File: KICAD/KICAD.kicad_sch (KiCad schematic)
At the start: 2327 parts, among them J3 Conn_02x20_Odd_Even, J4 Conn_01x02_Pin, J5 PJ-102A

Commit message: .
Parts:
- removed D2305, D2306, D2307, D2308, D2309, D2310, D2311, D2312, D2313, D2314, D2315, D2316, D2317, D2318, D2319, D2320, D2321, D2322, D2323, D2324, D2325, D2326, D2327, D2328, D2329, D2330, D2331, D2332, D2333, D2334, D2335, D2336, D2337, D2338, D2339, D2340, D2341, D2342, D2343, D2344, D2345, D2346, D2347, D2348, D2349, D2350, D2351, D2352, D2369, D2370, D2371, D2372, D2373, D2374, D2375, D2376, D2377, D2378, D2379, D2380, D2381, D2382, D2383, D2384, D2385, D2386, D2387, D2388, D2389, D2390, D2391, D2392, D2393, D2394, D2395, D2396, D2397, D2398, D2399, D2400, D2401, D2402, D2403, D2404, D2405, D2406, D2407, D2408, D2409, D2410, D2411, D2412, D2413, D2414, D2415, D2416, D2433, D2434, D2435, D2436, D2437, D2438, D2439, D2440, D2441, D2442, D2443, D2444, D2445, D2446, D2447, D2448, D2449, D2450, D2451, D2452, D2453, D2454, D2455, D2456, D2457, D2458, D2459, D2460, D2461, D2462, D2463, D2464, D2465, D2466, D2467, D2468, D2469, D2470, D2471, D2472, D2473, D2474, D2475, D2476, D2477, D2478, D2479, D2480, D2497, D2498, D2499, D2500, D2501, D2502, D2503, D2504, D2505, D2506, D2507, D2508, D2509, D2510, D2511, D2512, D2513, D2514, D2515, D2516, D2517, D2518, D2519, D2520, D2521, D2522, D2523, D2524, D2525, D2526, D2527, D2528, D2529, D2530, D2531, D2532, D2533, D2534, D2535, D2536, D2537, D2538, D2539, D2540, D2541, D2542, D2543, D2544, D2561, D2562, D2563, D2564, D2565, D2566, D2567, D2568, D2569, D2570, D2571, D2572, D2573, D2574, D2575, D2576, D2577, D2578, D2579, D2580, D2581, D2582, D2583, D2584, D2585, D2586, D2587, D2588, D2589, D2590, D2591, D2592, D2593, D2594, D2595, D2596, D2597, D2598, D2599, D2600, D2601, D2602, D2603, D2604, D2605, D2606, D2607, D2608, D2625, D2626, D2627, D2628, D2629, D2630, D2631, D2632, D2633, D2634, D2635, D2636, D2637, D2638, D2639, D2640, D2641, D2642, D2643, D2644, D2645, D2646, D2647, D2648, D2649, D2650, D2651, D2652, D2653, D2654, D2655, D2656, D2657, D2658, D2659, D2660, D2661, D2662, D2663, D2664, D2665, D2666, D2667, D2668, D2669, D2670, D2671, D2672, D2689, D2690, D2691, D2692, D2693, D2694, D2695, D2696, D2697, D2698, D2699, D2700, D2701, D2702, D2703, D2704, D2705, D2706, D2707, D2708, D2709, D2710, D2711, D2712, D2713, D2714, D2715, D2716, D2717, D2718, D2719, D2720, D2721, D2722, D2723, D2724, D2725, D2726, D2727, D2728, D2729, D2730, D2731, D2732, D2733, D2734, D2735, D2736, D2753, D2754, D2755, D2756, D2757, D2758, D2759, D2760, D2761, D2762, D2763, D2764, D2765, D2766, D2767, D2768, D2769, D2770, D2771, D2772, D2773, D2774, D2775, D2776, D2777, D2778, D2779, D2780, D2781, D2782, D2783, D2784, D2785, D2786, D2787, D2788, D2789, D2790, D2791, D2792, D2793, D2794, D2795, D2796, D2797, D2798, D2799, D2800, D2817, D2818, D2819, D2820, D2821, D2822, D2823, D2824, D2825, D2826, D2827, D2828, D2829, D2830, D2831, D2832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: WS2812B, LED_SMD:LED_WS2812B_PLCC4_5.0x5.0mm_P3.2mm, symbol LED:WS2812B
- removed J3: Conn_02x20_Odd_Even, Connector_IDC:IDC-Header_2x20_P2.54mm_Vertical_SMD, symbol Connector_Generic:Conn_02x20_Odd_Even
- added D1009, D1010, D1011, D1012, D1013, D1014, D1015, D1016, D1017, D1018, D1019, D1020, D1021, D1022, D1023, D1024, D1073, D1074, D1075, D1076, D1077, D1078, D1079, D1080, D1081, D1082, D1083, D1084, D1085, D1086, D1087, D1088, D113, D1137, D1138, D1139, D114, D1140, D1141, D1142, D1143, D1144, D1145, D1146, D1147, D1148, D1149, D115, D1150, D1151, D1152, D116, D117, D118, D119, D120, D1201, D1202, D1203, D1204, D1205, D1206, D1207, D1208, D1209, D121, D1210, D1211, D1212, D1213, D1214, D1215, D1216, D122, D123, D124, D125, D126, D1265, D1266, D1267, D1268, D1269, D127, D1270, D1271, D1272, D1273, D1274, D1275, D1276, D1277, D1278, D1279, D128, D1280, D1329, D1330, D1331, D1332, D1333, D1334, D1335, D1336, D1337, D1338, D1339, D1340, D1341, D1342, D1343, D1344, D1393, D1394, D1395, D1396, D1397, D1398, D1399, D1400, D1401, D1402, D1403, D1404, D1405, D1406, D1407, D1408, D1457, D1458, D1459, D1460, D1461, D1462, D1463, D1464, D1465, D1466, D1467, D1468, D1469, D1470, D1471, D1472, D1521, D1522, D1523, D1524, D1525, D1526, D1527, D1528, D1529, D1530, D1531, D1532, D1533, D1534, D1535, D1536, D1585, D1586, D1587, D1588, D1589, D1590, D1591, D1592, D1593, D1594, D1595, D1596, D1597, D1598, D1599, D1600, D1649, D1650, D1651, D1652, D1653, D1654, D1655, D1656, D1657, D1658, D1659, D1660, D1661, D1662, D1663, D1664, D1713, D1714, D1715, D1716, D1717, D1718, D1719, D1720, D1721, D1722, D1723, D1724, D1725, D1726, D1727, D1728, D177, D1777, D1778, D1779, D178, D1780, D1781, D1782, D1783, D1784, D1785, D1786, D1787, D1788, D1789, D179, D1790, D1791, D1792, D180, D181, D182, D183, D184, D1841, D1842, D1843, D1844, D1845, D1846, D1847, D1848, D1849, D185, D1850, D1851, D1852, D1853, D1854, D1855, D1856, D186, D187, D188, D189, D190, D1905, D1906, D1907, D1908, D1909, D191, D1910, D1911, D1912, D1913, D1914, D1915, D1916, D1917, D1918, D1919, D192, D1920, D1969, D1970, D1971, D1972, D1973, D1974, D1975, D1976, D1977, D1978, D1979, D1980, D1981, D1982, D1983, D1984, D2033, D2034, D2035, D2036, D2037, D2038, D2039, D2040, D2041, D2042, D2043, D2044, D2045, D2046, D2047, D2048, D2097, D2098, D2099, D2100, D2101, D2102, D2103, D2104, D2105, D2106, D2107, D2108, D2109, D2110, D2111, D2112, D2161, D2162, D2163, D2164, D2165, D2166, D2167, D2168, D2169, D2170, D2171, D2172, D2173, D2174, D2175, D2176, D2225, D2226, D2227, D2228, D2229, D2230, D2231, D2232, D2233, D2234, D2235, D2236, D2237, D2238, D2239, D2240, D2289, D2290, D2291, D2292, D2293, D2294, D2295, D2296, D2297, D2298, D2299, D2300, D2301, D2302, D2303, D2304, D241, D242, D243, D244, D245, D246, D247, D248, D249, D250, D251, D252, D253, D254, D255, D256, D305, D306, D307, D308, D309, D310, D311, D312, D313, D314, D315, D316, D317, D318, D319, D320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: WS2812B, LED_SMD:LED_WS2812B_PLCC4_5.0x5.0mm_P3.2mm, symbol LED:WS2812B
- added J3: Conn_02x25_Odd_Even, Connector_IDC:IDC-Header_2x25_P2.54mm_Vertical_SMD, symbol Connector_Generic:Conn_02x25_Odd_Even
- C1: footprint Capacitor_SMD:C_0603_1608Metric -> Capacitor_SMD:C_0402_1005Metric
- J5: footprint digikey-footprints:Barrel_Jack_5.5mmODx2.1mmID_PJ-102A -> Connector_BarrelJack:BarrelJack_Wuerth_694102107102_1.0x3.9mm
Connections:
- net BURST_A2 is gone; now on an unnamed net: D9.4 (DIN)
- net BURST_A3 is gone; now on an unnamed net: D17.4 (DIN)
- net BURST_A4 is gone; now on an unnamed net: D25.4 (DIN)
- net BURST_A5 is gone; now on an unnamed net: D33.4 (DIN)
- net BURST_A6 is gone; now on an unnamed net: D41.4 (DIN)
- net BURST_B5 is gone; now on an unnamed net: D545.4 (DIN)
- net BURST_B6 is gone; now on an unnamed net: D553.4 (DIN)
- net BURST_C3 is gone; now on an unnamed net: D1041.4 (DIN)
- net BURST_C4 is gone; now on an unnamed net: D1049.4 (DIN)
- net BURST_D2 is gone; now on an unnamed net: D1545.4 (DIN)
- net BURST_D3 is gone; now on an unnamed net: D1553.4 (DIN)
- net BURST_D4 is gone; now on an unnamed net: D1561.4 (DIN)
- net BURST_D6 is gone; now on an unnamed net: D1577.4 (DIN)
- net BURST_E2 is gone; now on an unnamed net: D2057.4 (DIN)
- net BURST_E4 is gone; now on an unnamed net: D2073.4 (DIN)
- net BURST_E5 is gone; now on an unnamed net: D2081.4 (DIN)
- net BURST_E6 is gone; now on an unnamed net: D2089.4 (DIN)
- net GND: now also D1009.3 (VSS), D1010.3 (VSS), D1011.3 (VSS), D1012.3 (VSS), D1013.3 (VSS), D1014.3 (VSS), D1015.3 (VSS), D1016.3 (VSS), D1017.3 (VSS), D1018.3 (VSS), D1019.3 (VSS), D1020.3 (VSS)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
- net VCC_3: now also D1009.1 (VDD), D1010.1 (VDD), D1011.1 (VDD), D1012.1 (VDD), D1013.1 (VDD), D1014.1 (VDD), D1015.1 (VDD), D1016.1 (VDD), D1017.1 (VDD), D1018.1 (VDD), D1019.1 (VDD), D1020.1 (VDD)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
- net at D1136.2 (DOUT): now also D1137.4 (DIN); no longer D1135.4 (DIN)
- net at D1072.2 (DOUT): now also D1073.4 (DIN); no longer D1136.4 (DIN)
- net at D1897.2 (DOUT): now also D1898.4 (DIN); no longer D1961.4 (DIN)
- net at D1897.4 (DIN): now also D1896.2 (DOUT); no longer D1898.2 (DOUT)
- net at D740.4 (DIN): now also D739.2 (DOUT); no longer D741.2 (DOUT)
- net at D742.2 (DOUT): now also D743.4 (DIN); no longer D741.4 (DIN)
- net at D364.4 (DIN): now also D363.2 (DOUT); no longer D365.2 (DOUT)
- net at D365.4 (DIN): now also D364.2 (DOUT); no longer D366.2 (DOUT)
- net at D1772.4 (DIN): now also D1771.2 (DOUT); no longer D1773.2 (DOUT)
- net at D1773.4 (DIN): now also D1772.2 (DOUT); no longer D1774.2 (DOUT)
- net at D607.2 (DOUT): now also D608.4 (DIN); no longer D606.4 (DIN)
- net at D607.4 (DIN): now also D606.2 (DOUT); no longer D608.2 (DOUT)
- net at D2270.4 (DIN): now also D2269.2 (DOUT); no longer D2271.2 (DOUT)
- net at D2272.2 (DOUT): now also D2273.4 (DIN); no longer D2271.4 (DIN)
- net at D2153.2 (DOUT): now also D2154.4 (DIN); no longer D2217.4 (DIN)
- net at D2153.4 (DIN): now also D2152.2 (DOUT); no longer D2154.2 (DOUT)
- net at D1740.2 (DOUT): now also D1741.4 (DIN); no longer D1739.4 (DIN)
- net at D1740.4 (DIN): now also D1739.2 (DOUT); no longer D1741.2 (DOUT)
- net at D665.4 (DIN): now also D664.2 (DOUT); no longer D601.2 (DOUT)
- net at D601.4 (DIN): now also D600.2 (DOUT); no longer D602.2 (DOUT)
- net at D100.2 (DOUT): now also D101.4 (DIN); no longer D99.4 (DIN)
- net at D101.2 (DOUT): now also D102.4 (DIN); no longer D100.4 (DIN)
- net at D1816.2 (DOUT): now also D1817.4 (DIN); no longer D1880.4 (DIN)
- net at D727.2 (DOUT): now also D728.4 (DIN); no longer D726.4 (DIN)
- net at D727.4 (DIN): now also D726.2 (DOUT); no longer D728.2 (DOUT)
- net at D1863.4 (DIN): now also D1862.2 (DOUT); no longer D1864.2 (DOUT)
- net at D1800.2 (DOUT): now also D1801.4 (DIN); no longer D1864.4 (DIN)
- net at D1874.2 (DOUT): now also D1875.4 (DIN); no longer D1873.4 (DIN)
- net at D1874.4 (DIN): now also D1873.2 (DOUT); no longer D1875.2 (DOUT)
- net at D196.2 (DOUT): now also D197.4 (DIN); no longer D195.4 (DIN)
- net at D197.2 (DOUT): now also D198.4 (DIN); no longer D196.4 (DIN)
- net at D2022.4 (DIN): now also D2021.2 (DOUT); no longer D2023.2 (DOUT)
- net at D2023.4 (DIN): now also D2022.2 (DOUT); no longer D2024.2 (DOUT)
- net at D617.4 (DIN): now also D616.2 (DOUT); no longer D618.2 (DOUT)
- net at D619.2 (DOUT): now also D620.4 (DIN); no longer D618.4 (DIN)
- net at D609.2 (DOUT): now also D610.4 (DIN); no longer D673.4 (DIN)
- net at D981.4 (DIN): now also D980.2 (DOUT); no longer D982.2 (DOUT)
- net at D982.4 (DIN): now also D981.2 (DOUT); no longer D983.2 (DOUT)
- net at D593.2 (DOUT): now also D594.4 (DIN); no longer D657.4 (DIN)
- net at D593.4 (DIN): now also D592.2 (DOUT); no longer D594.2 (DOUT)
- net at D905.4 (DIN): now also D904.2 (DOUT); no longer D841.2 (DOUT)
- net at D841.4 (DIN): now also D840.2 (DOUT); no longer D842.2 (DOUT)
- net at D1863.2 (DOUT): now also D1864.4 (DIN); no longer D1862.4 (DIN)
- net at D1387.2 (DOUT): now also D1388.4 (DIN); no longer D1386.4 (DIN)
- net at D1387.4 (DIN): now also D1386.2 (DOUT); no longer D1388.2 (DOUT)
- net at D230.2 (DOUT): now also D231.4 (DIN); no longer D229.4 (DIN)
- net at D231.2 (DOUT): now also D232.4 (DIN); no longer D230.4 (DIN)
- net at D860.4 (DIN): now also D859.2 (DOUT); no longer D861.2 (DOUT)
- net at D862.2 (DOUT): now also D863.4 (DIN); no longer D861.4 (DIN)
- net BURST_A1 renamed BURST_1
- net BURST_B3 renamed BURST_12
- net BURST_C5 renamed BURST_23
- net BURST_D1 renamed BURST_33
- net BURST_E3 renamed BURST_44
- new net: D1915.2 (DOUT), D1916.4 (DIN)
- new net: D1914.2 (DOUT), D1915.4 (DIN)
- new net: D441.2 (DOUT), D442.4 (DIN)
- new net: D440.2 (DOUT), D441.4 (DIN)
- new net: D1528.2 (DOUT), D1529.4 (DIN)
- new net: D1527.2 (DOUT), D1528.4 (DIN)
- new net: D435.2 (DOUT), D436.4 (DIN)
- new net: D434.2 (DOUT), D435.4 (DIN)
- new net: D694.2 (DOUT), D695.4 (DIN)
- new net: D693.2 (DOUT), D694.4 (DIN)
- new net: D2175.2 (DOUT), D2176.4 (DIN)
- new net: D2174.2 (DOUT), D2175.4 (DIN)
- new net: D628.2 (DOUT), D629.4 (DIN)
- new net: D627.2 (DOUT), D628.4 (DIN)
- new net: D1784.2 (DOUT), D1785.4 (DIN)
- new net: D1783.2 (DOUT), D1784.4 (DIN)
- new net: D2173.2 (DOUT), D2174.4 (DIN)
- new net: D2172.2 (DOUT), D2173.4 (DIN)
- new net: D1335.2 (DOUT), D1336.4 (DIN)
- new net: D1334.2 (DOUT), D1335.4 (DIN)
- new net: D509.2 (DOUT), D510.4 (DIN)
- new net: D508.2 (DOUT), D509.4 (DIN)
- new net: D433.2 (DOUT), D434.4 (DIN)
- new net: D49.2 (DOUT), D50.4 (DIN)
- new net: D1336.2 (DOUT), D1337.4 (DIN)
- new net: D1274.2 (DOUT), D1275.4 (DIN)
- new net: D1273.2 (DOUT), D1274.4 (DIN)
- new net: D1592.2 (DOUT), D1593.4 (DIN)
- new net: D1591.2 (DOUT), D1592.4 (DIN)
- new net: D1661.2 (DOUT), D1662.4 (DIN)
- new net: D1660.2 (DOUT), D1661.4 (DIN)
- new net: D1077.2 (DOUT), D1078.4 (DIN)
- new net: D1076.2 (DOUT), D1077.4 (DIN)
- new net: D753.2 (DOUT), D754.4 (DIN)
- new net: D59.2 (DOUT), D60.4 (DIN)
- new net: D58.2 (DOUT), D59.4 (DIN)
- new net: D370.2 (DOUT), D371.4 (DIN)
- new net: D369.2 (DOUT), D370.4 (DIN)
- new net: D1460.2 (DOUT), D1461.4 (DIN)
- new net: D1459.2 (DOUT), D1460.4 (DIN)
- new net: D1981.2 (DOUT), D1982.4 (DIN)
- new net: D1980.2 (DOUT), D1981.4 (DIN)
- new net: D767.2 (DOUT), D768.4 (DIN)
- new net: D766.2 (DOUT), D767.4 (DIN)
- new net: D1269.2 (DOUT), D1270.4 (DIN)
- new net: D1268.2 (DOUT), D1269.4 (DIN)
- new net: D1143.2 (DOUT), D1144.4 (DIN)
- new net: D1142.2 (DOUT), D1143.4 (DIN)
- new net: D1917.2 (DOUT), D1918.4 (DIN)
- new net: D1916.2 (DOUT), D1917.4 (DIN)
- new net: D639.2 (DOUT), D640.4 (DIN)
- new net: D638.2 (DOUT), D639.4 (DIN)
- new net: D1075.2 (DOUT), D1076.4 (DIN)
- new net: D1074.2 (DOUT), D1075.4 (DIN)
- new net: D1588.2 (DOUT), D1589.4 (DIN)
- new net: D1587.2 (DOUT), D1588.4 (DIN)
- new net: D1910.2 (DOUT), D1911.4 (DIN)
- new net: D1909.2 (DOUT), D1910.4 (DIN)
- new net: D1974.2 (DOUT), D1975.4 (DIN)
- new net: D1973.2 (DOUT), D1974.4 (DIN)
- new net: D894.2 (DOUT), D895.4 (DIN)
- new net: D893.2 (DOUT), D894.4 (DIN)
- new net: D1790.2 (DOUT), D1791.4 (DIN)
- new net: D1789.2 (DOUT), D1790.4 (DIN)
- new net: D182.2 (DOUT), D183.4 (DIN)
- new net: D181.2 (DOUT), D182.4 (DIN)
- new net: D1979.2 (DOUT), D1980.4 (DIN)
- new net: D1725.2 (DOUT), D1726.4 (DIN)
- new net: D1724.2 (DOUT), D1725.4 (DIN)
- new net: D2034.2 (DOUT), D2035.4 (DIN)
- new net: D2033.2 (DOUT), D2034.4 (DIN)
- new net: D1139.2 (DOUT), D1140.4 (DIN)
- new net: D1138.2 (DOUT), D1139.4 (DIN)
- new net: D114.2 (DOUT), D115.4 (DIN)
- new net: D113.2 (DOUT), D114.4 (DIN)
- new net: D1785.2 (DOUT), D1786.4 (DIN)
- new net: D500.2 (DOUT), D501.4 (DIN)
- new net: D499.2 (DOUT), D500.4 (DIN)
- new net: D1141.2 (DOUT), D1142.4 (DIN)
- new net: D1140.2 (DOUT), D1141.4 (DIN)
- new net: D507.2 (DOUT), D508.4 (DIN)
- new net: D568.2 (DOUT), D569.4 (DIN)
- new net: D567.2 (DOUT), D568.4 (DIN)
- new net: D881.2 (DOUT), D882.4 (DIN)
- new net: D1202.2 (DOUT), D1203.4 (DIN)
- new net: D1201.2 (DOUT), D1202.4 (DIN)
- new net: D1913.2 (DOUT), D1914.4 (DIN)
- new net: D1912.2 (DOUT), D1913.4 (DIN)
- new net: D820.2 (DOUT), D821.4 (DIN)
- new net: D819.2 (DOUT), D820.4 (DIN)
- new net: D1919.2 (DOUT), D1920.4 (DIN)
- new net: D2292.2 (DOUT), D2293.4 (DIN)
- new net: D2291.2 (DOUT), D2292.4 (DIN)
- new net: D1082.2 (DOUT), D1083.4 (DIN)
- new net: D1081.2 (DOUT), D1082.4 (DIN)
- new net: D243.2 (DOUT), D244.4 (DIN)
- new net: D242.2 (DOUT), D243.4 (DIN)
- new net: D1791.2 (DOUT), D1792.4 (DIN)
- new net: D689.2 (DOUT), D690.4 (DIN)
- new net: D2161.2 (DOUT), D2162.4 (DIN)
- new net: D1599.2 (DOUT), D1600.4 (DIN)
- new net: D1598.2 (DOUT), D1599.4 (DIN)
- new net: D1978.2 (DOUT), D1979.4 (DIN)
- new net: D1977.2 (DOUT), D1978.4 (DIN)
- new net: D1367.2 (DOUT), D1368.4 (DIN)
- new net: D762.2 (DOUT), D763.4 (DIN)
- new net: D761.2 (DOUT), D762.4 (DIN)
- new net: D2231.2 (DOUT), D2232.4 (DIN)
- new net: D2230.2 (DOUT), D2231.4 (DIN)
- new net: D1457.2 (DOUT), D1458.4 (DIN)
- new net: D1456.2 (DOUT), D1457.4 (DIN)
- new net: D1659.2 (DOUT), D1660.4 (DIN)
- new net: D1401.2 (DOUT), D1402.4 (DIN)
- new net: D1400.2 (DOUT), D1401.4 (DIN)
- new net: D888.2 (DOUT), D889.4 (DIN)
- new net: D887.2 (DOUT), D888.4 (DIN)
- new net: D191.2 (DOUT), D192.4 (DIN)
- new net: D190.2 (DOUT), D191.4 (DIN)
- new net: D1972.2 (DOUT), D1973.4 (DIN)
- new net: D631.2 (DOUT), D632.4 (DIN)
- new net: D630.2 (DOUT), D631.4 (DIN)
- new net: D1151.2 (DOUT), D1152.4 (DIN)
- new net: D1150.2 (DOUT), D1151.4 (DIN)
- new net: D1652.2 (DOUT), D1653.4 (DIN)
- new net: D1651.2 (DOUT), D1652.4 (DIN)
- new net: D377.2 (DOUT), D378.4 (DIN)
- new net: D376.2 (DOUT), D377.4 (DIN)
- new net: D1727.2 (DOUT), D1728.4 (DIN)
- new net: D1726.2 (DOUT), D1727.4 (DIN)
- new net: D700.2 (DOUT), D701.4 (DIN)
- new net: D699.2 (DOUT), D700.4 (DIN)
- new net: D51.2 (DOUT), D52.4 (DIN)
- new net: D50.2 (DOUT), D51.4 (DIN)
- new net: D255.2 (DOUT), D256.4 (DIN)
- new net: D254.2 (DOUT), D255.4 (DIN)
- new net: D572.2 (DOUT), D573.4 (DIN)
- new net: D571.2 (DOUT), D572.4 (DIN)
- new net: D2301.2 (DOUT), D2302.4 (DIN)
- new net: D2300.2 (DOUT), D2301.4 (DIN)
- new net: D245.2 (DOUT), D246.4 (DIN)
- new net: D244.2 (DOUT), D245.4 (DIN)
- new net: D1276.2 (DOUT), D1277.4 (DIN)
- new net: D1275.2 (DOUT), D1276.4 (DIN)
- new net: D252.2 (DOUT), D253.4 (DIN)
- new net: D251.2 (DOUT), D252.4 (DIN)
- new net: D946.2 (DOUT), D947.4 (DIN)
- new net: D945.2 (DOUT), D946.4 (DIN)
- new net: D2038.2 (DOUT), D2039.4 (DIN)
- new net: D2037.2 (DOUT), D2038.4 (DIN)
- new net: D1396.2 (DOUT), D1397.4 (DIN)
- new net: D1395.2 (DOUT), D1396.4 (DIN)
- new net: D1969.2 (DOUT), D1970.4 (DIN)
- new net: D317.2 (DOUT), D318.4 (DIN)
- new net: D316.2 (DOUT), D317.4 (DIN)
- new net: D1085.2 (DOUT), D1086.4 (DIN)
- new net: D1084.2 (DOUT), D1085.4 (DIN)
- new net: D1786.2 (DOUT), D1787.4 (DIN)
- new net: D1533.2 (DOUT), D1534.4 (DIN)
- new net: D1532.2 (DOUT), D1533.4 (DIN)
- new net: D1653.2 (DOUT), D1654.4 (DIN)
- new net: D574.2 (DOUT), D575.4 (DIN)
- new net: D573.2 (DOUT), D574.4 (DIN)
- new net: D702.2 (DOUT), D703.4 (DIN)
- new net: D701.2 (DOUT), D702.4 (DIN)
- new net: D320.2 (DOUT), D321.4 (DIN)
- new net: D319.2 (DOUT), D320.4 (DIN)
- new net: D1018.2 (DOUT), D1019.4 (DIN)
- new net: D1017.2 (DOUT), D1018.4 (DIN)
- new net: D1777.2 (DOUT), D1778.4 (DIN)
- new net: D634.2 (DOUT), D635.4 (DIN)
- new net: D633.2 (DOUT), D634.4 (DIN)
- new net: D379.2 (DOUT), D380.4 (DIN)
- new net: D378.2 (DOUT), D379.4 (DIN)
- new net: D188.2 (DOUT), D189.4 (DIN)
- new net: D187.2 (DOUT), D188.4 (DIN)
- new net: D1011.2 (DOUT), D1012.4 (DIN)
- new net: D1010.2 (DOUT), D1011.4 (DIN)
- new net: D502.2 (DOUT), D503.4 (DIN)
- new net: D501.2 (DOUT), D502.4 (DIN)
- new net: D2035.2 (DOUT), D2036.4 (DIN)
- new net: D1535.2 (DOUT), D1536.4 (DIN)
- new net: D1083.2 (DOUT), D1084.4 (DIN)
- new net: D1713.2 (DOUT), D1714.4 (DIN)
- new net: D1023.2 (DOUT), D1024.4 (DIN)
- new net: D1022.2 (DOUT), D1023.4 (DIN)
- new net: D2110.2 (DOUT), D2111.4 (DIN)
- new net: D2109.2 (DOUT), D2110.4 (DIN)
- new net: D1656.2 (DOUT), D1657.4 (DIN)
- new net: D1655.2 (DOUT), D1656.4 (DIN)
- new net: D1342.2 (DOUT), D1343.4 (DIN)
- new net: D1341.2 (DOUT), D1342.4 (DIN)
- new net: D765.2 (DOUT), D766.4 (DIN)
- new net: D764.2 (DOUT), D765.4 (DIN)
- new net: D823.2 (DOUT), D824.4 (DIN)
- new net: D822.2 (DOUT), D823.4 (DIN)
- new net: D1137.2 (DOUT), D1138.4 (DIN)
- new net: D1271.2 (DOUT), D1272.4 (DIN)
- new net: D1270.2 (DOUT), D1271.4 (DIN)
- new net: D307.2 (DOUT), D308.4 (DIN)
- new net: D306.2 (DOUT), D307.4 (DIN)
- new net: D444.2 (DOUT), D445.4 (DIN)
- new net: D443.2 (DOUT), D444.4 (DIN)
- new net: D2162.2 (DOUT), D2163.4 (DIN)
- new net: D1593.2 (DOUT), D1594.4 (DIN)
- new net: D116.2 (DOUT), D117.4 (DIN)
- new net: D115.2 (DOUT), D116.4 (DIN)
- new net: D697.2 (DOUT), D698.4 (DIN)
- new net: D696.2 (DOUT), D697.4 (DIN)
- new net: D57.2 (DOUT), D58.4 (DIN)
- new net: D54.2 (DOUT), D55.4 (DIN)
- new net: D53.2 (DOUT), D54.4 (DIN)
- new net: D1970.2 (DOUT), D1971.4 (DIN)
- new net: D691.2 (DOUT), D692.4 (DIN)
- new net: D690.2 (DOUT), D691.4 (DIN)
- new net: D896.2 (DOUT), D897.4 (DIN)
- new net: D740.2 (DOUT), D741.4 (DIN)
- new net: D1754.2 (DOUT), D1755.4 (DIN)
- new net: D1975.2 (DOUT), D1976.4 (DIN)
- new net: D1339.2 (DOUT), D1340.4 (DIN)
- new net: D1338.2 (DOUT), D1339.4 (DIN)
- new net: D886.2 (DOUT), D887.4 (DIN)
- new net: D885.2 (DOUT), D886.4 (DIN)
- new net: D2108.2 (DOUT), D2109.4 (DIN)
- new net: D2107.2 (DOUT), D2108.4 (DIN)
- new net: D884.2 (DOUT), D885.4 (DIN)
- new net: D2232.2 (DOUT), D2233.4 (DIN)
- new net: D2036.2 (DOUT), D2037.4 (DIN)
- new net: D2236.2 (DOUT), D2237.4 (DIN)
- new net: D2235.2 (DOUT), D2236.4 (DIN)
- new net: D1021.2 (DOUT), D1022.4 (DIN)
- new net: D1842.2 (DOUT), D1843.4 (DIN)
- new net: D1841.2 (DOUT), D1842.4 (DIN)
- new net: D1715.2 (DOUT), D1716.4 (DIN)
- new net: D1714.2 (DOUT), D1715.4 (DIN)
- new net: D1983.2 (DOUT), D1984.4 (DIN)
- new net: D1982.2 (DOUT), D1983.4 (DIN)
- new net: D1337.2 (DOUT), D1338.4 (DIN)
- new net: D569.2 (DOUT), D570.4 (DIN)
- new net: D383.2 (DOUT), D384.4 (DIN)
- new net: D703.2 (DOUT), D704.4 (DIN)
- new net: D1272.2 (DOUT), D1273.4 (DIN)
- new net: D1206.2 (DOUT), D1207.4 (DIN)
- new net: D1205.2 (DOUT), D1206.4 (DIN)
- new net: D52.2 (DOUT), D53.4 (DIN)
- new net: D250.2 (DOUT), D251.4 (DIN)
- new net: D1215.2 (DOUT), D1216.4 (DIN)
- new net: D1214.2 (DOUT), D1215.4 (DIN)
- new net: D511.2 (DOUT), D512.4 (DIN)
- new net: D510.2 (DOUT), D511.4 (DIN)
- new net: D2303.2 (DOUT), D2304.4 (DIN)
- new net: D2302.2 (DOUT), D2303.4 (DIN)
- new net: D305.2 (DOUT), D306.4 (DIN)
- new net: D1531.2 (DOUT), D1532.4 (DIN)
- new net: D1530.2 (DOUT), D1531.4 (DIN)
- new net: D695.2 (DOUT), D696.4 (DIN)
- new net: D1534.2 (DOUT), D1535.4 (DIN)
- new net: D118.2 (DOUT), D119.4 (DIN)
- new net: D117.2 (DOUT), D118.4 (DIN)
- new net: D372.2 (DOUT), D373.4 (DIN)
- new net: D371.2 (DOUT), D372.4 (DIN)
- new net: D1905.2 (DOUT), D1906.4 (DIN)
- new net: D436.2 (DOUT), D437.4 (DIN)
- new net: D1851.2 (DOUT), D1852.4 (DIN)
- new net: D1850.2 (DOUT), D1851.4 (DIN)
- new net: D1403.2 (DOUT), D1404.4 (DIN)
- new net: D1402.2 (DOUT), D1403.4 (DIN)
- new net: D1458.2 (DOUT), D1459.4 (DIN)
- new net: D829.2 (DOUT), D830.4 (DIN)
- new net: D828.2 (DOUT), D829.4 (DIN)
- new net: D1852.2 (DOUT), D1853.4 (DIN)
- new net: D1918.2 (DOUT), D1919.4 (DIN)
- new net: D1986.2 (DOUT), D1987.4 (DIN)
- new net: D763.2 (DOUT), D764.4 (DIN)
- new net: D1657.2 (DOUT), D1658.4 (DIN)
- new net: D1404.2 (DOUT), D1405.4 (DIN)
- new net: D189.2 (DOUT), D190.4 (DIN)
- new net: D382.2 (DOUT), D383.4 (DIN)
- new net: D381.2 (DOUT), D382.4 (DIN)
- new net: D1516.2 (DOUT), D1517.4 (DIN)
- new net: D2105.2 (DOUT), D2106.4 (DIN)
- new net: D2104.2 (DOUT), D2105.4 (DIN)
- new net: D122.2 (DOUT), D123.4 (DIN)
- new net: D121.2 (DOUT), D122.4 (DIN)
- new net: D1662.2 (DOUT), D1663.4 (DIN)
- new net: D1333.2 (DOUT), D1334.4 (DIN)
- new net: D1332.2 (DOUT), D1333.4 (DIN)
- new net: D564.2 (DOUT), D565.4 (DIN)
- new net: D563.2 (DOUT), D564.4 (DIN)
- new net: D180.2 (DOUT), D181.4 (DIN)
- new net: D2295.2 (DOUT), D2296.4 (DIN)
- new net: D2294.2 (DOUT), D2295.4 (DIN)
- new net: D2169.2 (DOUT), D2170.4 (DIN)
- new net: D2168.2 (DOUT), D2169.4 (DIN)
- new net: D2133.2 (DOUT), D2134.4 (DIN)
- new net: D959.2 (DOUT), D960.4 (DIN)
- new net: D958.2 (DOUT), D959.4 (DIN)
- new net: D2045.2 (DOUT), D2046.4 (DIN)
- new net: D2044.2 (DOUT), D2045.4 (DIN)
- new net: D315.2 (DOUT), D316.4 (DIN)
- new net: D314.2 (DOUT), D315.4 (DIN)
- new net: D1279.2 (DOUT), D1280.4 (DIN)
- new net: D1278.2 (DOUT), D1279.4 (DIN)
- new net: D1212.2 (DOUT), D1213.4 (DIN)
- new net: D1211.2 (DOUT), D1212.4 (DIN)
- new net: D1080.2 (DOUT), D1081.4 (DIN)
- new net: D635.2 (DOUT), D636.4 (DIN)
- new net: D751.2 (DOUT), D752.4 (DIN)
- new net: D1213.2 (DOUT), D1214.4 (DIN)
- new net: D445.2 (DOUT), D446.4 (DIN)
- new net: D566.2 (DOUT), D567.4 (DIN)
- new net: D505.2 (DOUT), D506.4 (DIN)
- new net: D504.2 (DOUT), D505.4 (DIN)
- new net: D1506.2 (DOUT), D1507.4 (DIN)
- new net: D1020.2 (DOUT), D1021.4 (DIN)
- new net: D1529.2 (DOUT), D1530.4 (DIN)
- new net: D253.2 (DOUT), D254.4 (DIN)
- new net: D1340.2 (DOUT), D1341.4 (DIN)
- new net: D491.2 (DOUT), D492.4 (DIN)
- new net: D490.2 (DOUT), D491.4 (DIN)
- new net: D1782.2 (DOUT), D1783.4 (DIN)
- new net: D1781.2 (DOUT), D1782.4 (DIN)
- new net: D2234.2 (DOUT), D2235.4 (DIN)
- new net: D2233.2 (DOUT), D2234.4 (DIN)
- new net: D1911.2 (DOUT), D1912.4 (DIN)
- new net: D892.2 (DOUT), D893.4 (DIN)
- new net: D1779.2 (DOUT), D1780.4 (DIN)
- new net: D1778.2 (DOUT), D1779.4 (DIN)
- new net: D2163.2 (DOUT), D2164.4 (DIN)
- new net: D1086.2 (DOUT), D1087.4 (DIN)
- new net: D120.2 (DOUT), D121.4 (DIN)
- new net: D119.2 (DOUT), D120.4 (DIN)
- new net: D994.2 (DOUT), D995.4 (DIN)
- new net: D484.2 (DOUT), D485.4 (DIN)
- new net: D1407.2 (DOUT), D1408.4 (DIN)
- new net: D1406.2 (DOUT), D1407.4 (DIN)
- new net: D2246.2 (DOUT), D2247.4 (DIN)
- new net: D1526.2 (DOUT), D1527.4 (DIN)
- new net: D951.2 (DOUT), D952.4 (DIN)
- new net: D950.2 (DOUT), D951.4 (DIN)
- new net: D61.2 (DOUT), D62.4 (DIN)
- new net: D60.2 (DOUT), D61.4 (DIN)
- new net: D2039.2 (DOUT), D2040.4 (DIN)
- new net: D483.2 (DOUT), D484.4 (DIN)
- new net: D2247.2 (DOUT), D2248.4 (DIN)
- new net: D309.2 (DOUT), D310.4 (DIN)
- new net: D308.2 (DOUT), D309.4 (DIN)
- new net: D876.2 (DOUT), D877.4 (DIN)
- new net: D891.2 (DOUT), D892.4 (DIN)
- new net: D890.2 (DOUT), D891.4 (DIN)
- new net: D1399.2 (DOUT), D1400.4 (DIN)
- new net: D560.2 (DOUT), D561.4 (DIN)
- new net: D152.2 (DOUT), D153.4 (DIN)
- new net: D889.2 (DOUT), D890.4 (DIN)
- new net: D2149.2 (DOUT), D2150.4 (DIN)
- new net: D2226.2 (DOUT), D2227.4 (DIN)
- new net: D2225.2 (DOUT), D2226.4 (DIN)
- new net: D875.2 (DOUT), D876.4 (DIN)
- new net: D2293.2 (DOUT), D2294.4 (DIN)
- new net: D1525.2 (DOUT), D1526.4 (DIN)
- new net: D1524.2 (DOUT), D1525.4 (DIN)
- new net: D1471.2 (DOUT), D1472.4 (DIN)
- new net: D1470.2 (DOUT), D1471.4 (DIN)
- new net: D1898.2 (DOUT), D1899.4 (DIN)
- new net: D56.2 (DOUT), D57.4 (DIN)
- new net: D55.2 (DOUT), D56.4 (DIN)
- new net: D1637.2 (DOUT), D1638.4 (DIN)
- new net: D1370.2 (DOUT), D1371.4 (DIN)
- new net: D620.2 (DOUT), D621.4 (DIN)
- new net: D1788.2 (DOUT), D1789.4 (DIN)
- new net: D1787.2 (DOUT), D1788.4 (DIN)
- new net: D503.2 (DOUT), D504.4 (DIN)
- new net: D1227.2 (DOUT), D1228.4 (DIN)
- new net: D2043.2 (DOUT), D2044.4 (DIN)
- new net: D2042.2 (DOUT), D2043.4 (DIN)
- new net: D947.2 (DOUT), D948.4 (DIN)
- new net: D1087.2 (DOUT), D1088.4 (DIN)
- new net: D882.2 (DOUT), D883.4 (DIN)
- new net: D1720.2 (DOUT), D1721.4 (DIN)
- new net: D1719.2 (DOUT), D1720.4 (DIN)
- new net: D239.2 (DOUT), D240.4 (DIN)
- new net: D437.2 (DOUT), D438.4 (DIN)
- new net: D2099.2 (DOUT), D2100.4 (DIN)
- new net: D2098.2 (DOUT), D2099.4 (DIN)
- new net: D1595.2 (DOUT), D1596.4 (DIN)
- new net: D1594.2 (DOUT), D1595.4 (DIN)
- new net: D953.2 (DOUT), D954.4 (DIN)
- new net: D952.2 (DOUT), D953.4 (DIN)
- new net: D179.2 (DOUT), D180.4 (DIN)
- new net: D178.2 (DOUT), D179.4 (DIN)
- new net: D821.2 (DOUT), D822.4 (DIN)
- new net: D1971.2 (DOUT), D1972.4 (DIN)
- new net: D83.2 (DOUT), D84.4 (DIN)
- new net: D2238.2 (DOUT), D2239.4 (DIN)
- new net: D2237.2 (DOUT), D2238.4 (DIN)
- new net: D2103.2 (DOUT), D2104.4 (DIN)
- new net: D2102.2 (DOUT), D2103.4 (DIN)
- new net: D79.2 (DOUT), D80.4 (DIN)
- new net: D975.2 (DOUT), D976.4 (DIN)
- new net: D1465.2 (DOUT), D1466.4 (DIN)
- new net: D1464.2 (DOUT), D1465.4 (DIN)
- new net: D2299.2 (DOUT), D2300.4 (DIN)
- new net: D2298.2 (DOUT), D2299.4 (DIN)
- new net: D2171.2 (DOUT), D2172.4 (DIN)
- new net: D1073.2 (DOUT), D1074.4 (DIN)
- new net: D1746.2 (DOUT), D1747.4 (DIN)
- new net: D755.2 (DOUT), D756.4 (DIN)
- new net: D754.2 (DOUT), D755.4 (DIN)
- new net: D463.2 (DOUT), D464.4 (DIN)
- new net: D78.2 (DOUT), D79.4 (DIN)
- new net: D1757.2 (DOUT), D1758.4 (DIN)
- new net: D63.2 (DOUT), D64.4 (DIN)
- new net: D62.2 (DOUT), D63.4 (DIN)
- new net: D2239.2 (DOUT), D2240.4 (DIN)
- new net: D858.2 (DOUT), D859.4 (DIN)
- new net: D1486.2 (DOUT), D1487.4 (DIN)
- new net: D1883.2 (DOUT), D1884.4 (DIN)
- new net: D1654.2 (DOUT), D1655.4 (DIN)
- new net: D1148.2 (DOUT), D1149.4 (DIN)
- new net: D1147.2 (DOUT), D1148.4 (DIN)
- new net: D2284.2 (DOUT), D2285.4 (DIN)
- new net: D374.2 (DOUT), D375.4 (DIN)
- new net: D373.2 (DOUT), D374.4 (DIN)
- new net: D1009.2 (DOUT), D1010.4 (DIN)
- new net: D126.2 (DOUT), D127.4 (DIN)
- new net: D125.2 (DOUT), D126.4 (DIN)
- new net: D625.2 (DOUT), D626.4 (DIN)
- new net: D506.2 (DOUT), D507.4 (DIN)
- new net: D1844.2 (DOUT), D1845.4 (DIN)
- new net: D1843.2 (DOUT), D1844.4 (DIN)
- new net: D757.2 (DOUT), D758.4 (DIN)
- new net: D756.2 (DOUT), D757.4 (DIN)
- new net: D1234.2 (DOUT), D1235.4 (DIN)
- new net: D605.2 (DOUT), D606.4 (DIN)
- new net: D883.2 (DOUT), D884.4 (DIN)
- new net: D1716.2 (DOUT), D1717.4 (DIN)
- new net: D632.2 (DOUT), D633.4 (DIN)
- new net: D2097.2 (DOUT), D2098.4 (DIN)
- new net: D1145.2 (DOUT), D1146.4 (DIN)
- new net: D1144.2 (DOUT), D1145.4 (DIN)
- new net: D246.2 (DOUT), D247.4 (DIN)
- new net: D895.2 (DOUT), D896.4 (DIN)
- new net: D1216.2 (DOUT), D1217.4 (DIN)
- new net: D728.2 (DOUT), D729.4 (DIN)
- new net: D2100.2 (DOUT), D2101.4 (DIN)
- new net: D1398.2 (DOUT), D1399.4 (DIN)
- new net: D1079.2 (DOUT), D1080.4 (DIN)
- new net: D1331.2 (DOUT), D1332.4 (DIN)
- new net: D1330.2 (DOUT), D1331.4 (DIN)
- new net: D1130.2 (DOUT), D1131.4 (DIN)
- new net: D2008.2 (DOUT), D2009.4 (DIN)
- new net: D1721.2 (DOUT), D1722.4 (DIN)
- new net: D1014.2 (DOUT), D1015.4 (DIN)
- new net: D1013.2 (DOUT), D1014.4 (DIN)
- new net: D565.2 (DOUT), D566.4 (DIN)
- new net: D2227.2 (DOUT), D2228.4 (DIN)
- new net: D957.2 (DOUT), D958.4 (DIN)
- new net: D956.2 (DOUT), D957.4 (DIN)
- new net: D1780.2 (DOUT), D1781.4 (DIN)
- new net: D71.2 (DOUT), D72.4 (DIN)
- new net: D1146.2 (DOUT), D1147.4 (DIN)
- new net: D2007.2 (DOUT), D2008.4 (DIN)
- new net: D1255.2 (DOUT), D1256.4 (DIN)
- new net: D1856.2 (DOUT), D1857.4 (DIN)
- new net: D1855.2 (DOUT), D1856.4 (DIN)
- new net: D954.2 (DOUT), D955.4 (DIN)
- new net: D110.2 (DOUT), D111.4 (DIN)
- new net: D2040.2 (DOUT), D2041.4 (DIN)
- new net: D304.2 (DOUT), D305.4 (DIN)
- new net: D1485.2 (DOUT), D1486.4 (DIN)
- new net: D455.2 (DOUT), D456.4 (DIN)
- new net: D1522.2 (DOUT), D1523.4 (DIN)
- new net: D1521.2 (DOUT), D1522.4 (DIN)
- new net: D2119.2 (DOUT), D2120.4 (DIN)
- new net: D310.2 (DOUT), D311.4 (DIN)
- new net: D577.2 (DOUT), D578.4 (DIN)
- new net: D1886.2 (DOUT), D1887.4 (DIN)
- new net: D949.2 (DOUT), D950.4 (DIN)
- new net: D296.2 (DOUT), D297.4 (DIN)
- new net: D1203.2 (DOUT), D1204.4 (DIN)
- new net: D1523.2 (DOUT), D1524.4 (DIN)
- new net: D2047.2 (DOUT), D2048.4 (DIN)
- new net: D2046.2 (DOUT), D2047.4 (DIN)
- new net: D1397.2 (DOUT), D1398.4 (DIN)
- new net: D1847.2 (DOUT), D1848.4 (DIN)
- new net: D1846.2 (DOUT), D1847.4 (DIN)
- new net: D1808.2 (DOUT), D1809.4 (DIN)
- new net: D692.2 (DOUT), D693.4 (DIN)
- new net: D743.2 (DOUT), D744.4 (DIN)
- new net: D1016.2 (DOUT), D1017.4 (DIN)
- new net: D1015.2 (DOUT), D1016.4 (DIN)
- new net: D2167.2 (DOUT), D2168.4 (DIN)
- new net: D2166.2 (DOUT), D2167.4 (DIN)
- new net: D626.2 (DOUT), D627.4 (DIN)
- new net: D948.2 (DOUT), D949.4 (DIN)
- new net: D1589.2 (DOUT), D1590.4 (DIN)
- new net: D238.2 (DOUT), D239.4 (DIN)
- new net: D318.2 (DOUT), D319.4 (DIN)
- new net: D1762.2 (DOUT), D1763.4 (DIN)
- new net: D986.2 (DOUT), D987.4 (DIN)
- new net: D2041.2 (DOUT), D2042.4 (DIN)
- new net: D2296.2 (DOUT), D2297.4 (DIN)
- new net: D1854.2 (DOUT), D1855.4 (DIN)
- new net: D1853.2 (DOUT), D1854.4 (DIN)
- new net: D719.2 (DOUT), D720.4 (DIN)
- new net: D1864.2 (DOUT), D1865.4 (DIN)
- new net: D561.2 (DOUT), D562.4 (DIN)
- new net: D2128.2 (DOUT), D2129.4 (DIN)
- new net: D852.2 (DOUT), D853.4 (DIN)
- new net: D1463.2 (DOUT), D1464.4 (DIN)
- new net: D712.2 (DOUT), D713.4 (DIN)
- new net: D1405.2 (DOUT), D1406.4 (DIN)
- new net: D460.2 (DOUT), D461.4 (DIN)
- new net: D2297.2 (DOUT), D2298.4 (DIN)
- new net: D832.2 (DOUT), D833.4 (DIN)
- new net: D1245.2 (DOUT), D1246.4 (DIN)
- new net: D1007.2 (DOUT), D1008.4 (DIN)
- new net: D1849.2 (DOUT), D1850.4 (DIN)
- new net: D1848.2 (DOUT), D1849.4 (DIN)
- new net: D1123.2 (DOUT), D1124.4 (DIN)
- new net: D1088.2 (DOUT), D1089.4 (DIN)
- new net: D1774.2 (DOUT), D1775.4 (DIN)
- new net: D1019.2 (DOUT), D1020.4 (DIN)
- new net: D1383.2 (DOUT), D1384.4 (DIN)
- new net: D313.2 (DOUT), D314.4 (DIN)
- new net: D562.2 (DOUT), D563.4 (DIN)
- new net: D629.2 (DOUT), D630.4 (DIN)
- new net: D2157.2 (DOUT), D2158.4 (DIN)
- new net: D974.2 (DOUT), D975.4 (DIN)
- new net: D325.2 (DOUT), D326.4 (DIN)
- new net: D1976.2 (DOUT), D1977.4 (DIN)
- new net: D1612.2 (DOUT), D1613.4 (DIN)
- new net: D1356.2 (DOUT), D1357.4 (DIN)
- new net: D127.2 (DOUT), D128.4 (DIN)
- new net: D826.2 (DOUT), D827.4 (DIN)
- new net: D825.2 (DOUT), D826.4 (DIN)
- new net: D1210.2 (DOUT), D1211.4 (DIN)
- new net: D1209.2 (DOUT), D1210.4 (DIN)
- new net: D1664.2 (DOUT), D1665.4 (DIN)
- new net: D824.2 (DOUT), D825.4 (DIN)
- new net: D248.2 (DOUT), D249.4 (DIN)
- new net: D247.2 (DOUT), D248.4 (DIN)
- new net: D1618.2 (DOUT), D1619.4 (DIN)
- new net: D368.2 (DOUT), D369.4 (DIN)
- new net: D1462.2 (DOUT), D1463.4 (DIN)
- new net: D1394.2 (DOUT), D1395.4 (DIN)
- new net: D1765.2 (DOUT), D1766.4 (DIN)
- new net: D475.2 (DOUT), D476.4 (DIN)
- new net: D474.2 (DOUT), D475.4 (DIN)
- new net: D1267.2 (DOUT), D1268.4 (DIN)
- new net: D1078.2 (DOUT), D1079.4 (DIN)
- new net: D351.2 (DOUT), D352.4 (DIN)
- new net: D160.2 (DOUT), D161.4 (DIN)
- new net: D1122.2 (DOUT), D1123.4 (DIN)
- new net: D1597.2 (DOUT), D1598.4 (DIN)
- new net: D1596.2 (DOUT), D1597.4 (DIN)
- new net: D706.2 (DOUT), D707.4 (DIN)
- new net: D1149.2 (DOUT), D1150.4 (DIN)
- new net: D1602.2 (DOUT), D1603.4 (DIN)
- new net: D224.2 (DOUT), D225.4 (DIN)
- new net: D1348.2 (DOUT), D1349.4 (DIN)
- new net: D2144.2 (DOUT), D2145.4 (DIN)
- new net: D2143.2 (DOUT), D2144.4 (DIN)
- new net: D1277.2 (DOUT), D1278.4 (DIN)
- new net: D375.2 (DOUT), D376.4 (DIN)
- new net: D350.2 (DOUT), D351.4 (DIN)
- new net: D177.2 (DOUT), D178.4 (DIN)
- new net: D1585.2 (DOUT), D1586.4 (DIN)
- new net: D195.2 (DOUT), D196.4 (DIN)
- new net: D759.2 (DOUT), D760.4 (DIN)
- new net: D758.2 (DOUT), D759.4 (DIN)
- new net: D2290.2 (DOUT), D2291.4 (DIN)
- new net: D2289.2 (DOUT), D2290.4 (DIN)
- new net: D997.2 (DOUT), D998.4 (DIN)
- new net: D439.2 (DOUT), D440.4 (DIN)
- new net: D333.2 (DOUT), D334.4 (DIN)
- new net: D1108.2 (DOUT), D1109.4 (DIN)
- new net: D1249.2 (DOUT), D1250.4 (DIN)
- new net: D1466.2 (DOUT), D1467.4 (DIN)
- new net: D1266.2 (DOUT), D1267.4 (DIN)
- new net: D2024.2 (DOUT), D2025.4 (DIN)
- new net: D1658.2 (DOUT), D1659.4 (DIN)
- new net: D1480.2 (DOUT), D1481.4 (DIN)
- new net: D1718.2 (DOUT), D1719.4 (DIN)
- new net: D1717.2 (DOUT), D1718.4 (DIN)
- new net: D1875.2 (DOUT), D1876.4 (DIN)
- new net: D637.2 (DOUT), D638.4 (DIN)
- new net: D636.2 (DOUT), D637.4 (DIN)
- new net: D2027.2 (DOUT), D2028.4 (DIN)
- new net: D380.2 (DOUT), D381.4 (DIN)
- new net: D1135.2 (DOUT), D1136.4 (DIN)
- new net: D1586.2 (DOUT), D1587.4 (DIN)
- new net: D831.2 (DOUT), D832.4 (DIN)
- new net: D1773.2 (DOUT), D1774.4 (DIN)
- new net: D867.2 (DOUT), D868.4 (DIN)
- new net: D249.2 (DOUT), D250.4 (DIN)
- new net: D203.2 (DOUT), D204.4 (DIN)
- new net: D497.2 (DOUT), D498.4 (DIN)
- new net: D1688.2 (DOUT), D1689.4 (DIN)
- new net: D1393.2 (DOUT), D1394.4 (DIN)
- new net: D1204.2 (DOUT), D1205.4 (DIN)
- new net: D1623.2 (DOUT), D1624.4 (DIN)
- new net: D64.2 (DOUT), D65.4 (DIN)
- new net: D1590.2 (DOUT), D1591.4 (DIN)
- new net: D1952.2 (DOUT), D1953.4 (DIN)
- new net: D1114.2 (DOUT), D1115.4 (DIN)
- new net: D442.2 (DOUT), D443.4 (DIN)
- new net: D760.2 (DOUT), D761.4 (DIN)
- new net: D575.2 (DOUT), D576.4 (DIN)
- new net: D123.2 (DOUT), D124.4 (DIN)
- new net: D1105.2 (DOUT), D1106.4 (DIN)
- new net: D2101.2 (DOUT), D2102.4 (DIN)
- new net: D1903.2 (DOUT), D1904.4 (DIN)
- new net: D817.2 (DOUT), D818.4 (DIN)
- new net: D2170.2 (DOUT), D2171.4 (DIN)
- new net: D1208.2 (DOUT), D1209.4 (DIN)
- new net: D1207.2 (DOUT), D1208.4 (DIN)
- new net: D1907.2 (DOUT), D1908.4 (DIN)
- new net: D1906.2 (DOUT), D1907.4 (DIN)
- new net: D1722.2 (DOUT), D1723.4 (DIN)
- new net: D334.2 (DOUT), D335.4 (DIN)
- new net: D186.2 (DOUT), D187.4 (DIN)
- new net: D498.2 (DOUT), D499.4 (DIN)
- new net: D1467.2 (DOUT), D1468.4 (DIN)
- new net: D2266.2 (DOUT), D2267.4 (DIN)
- new net: D1343.2 (DOUT), D1344.4 (DIN)
- new net: D987.2 (DOUT), D988.4 (DIN)
- new net: D312.2 (DOUT), D313.4 (DIN)
- new net: D311.2 (DOUT), D312.4 (DIN)
- new net: D128.2 (DOUT), D129.4 (DIN)
- new net: D2106.2 (DOUT), D2107.4 (DIN)
- new net: D2111.2 (DOUT), D2112.4 (DIN)
- new net: D1280.2 (DOUT), D1281.4 (DIN)
- new net: D1012.2 (DOUT), D1013.4 (DIN)
- new net: D1468.2 (DOUT), D1469.4 (DIN)
- new net: D1265.2 (DOUT), D1266.4 (DIN)
- new net: D1264.2 (DOUT), D1265.4 (DIN)
- new net: D827.2 (DOUT), D828.4 (DIN)
- new net: D570.2 (DOUT), D571.4 (DIN)
- new net: D2263.2 (DOUT), D2264.4 (DIN)
- new net: D1663.2 (DOUT), D1664.4 (DIN)
- new net: D818.2 (DOUT), D819.4 (DIN)
- new net: D1119.2 (DOUT), D1120.4 (DIN)
- new net: D1723.2 (DOUT), D1724.4 (DIN)
- new net: D1650.2 (DOUT), D1651.4 (DIN)
- new net: D1649.2 (DOUT), D1650.4 (DIN)
- new net: D2165.2 (DOUT), D2166.4 (DIN)
- new net: D2164.2 (DOUT), D2165.4 (DIN)
- new net: D72.2 (DOUT), D73.4 (DIN)
- new net: D1845.2 (DOUT), D1846.4 (DIN)
- new net: D721.2 (DOUT), D722.4 (DIN)
- new net: D830.2 (DOUT), D831.4 (DIN)
- new net: D843.2 (DOUT), D844.4 (DIN)
- new net: D241.2 (DOUT), D242.4 (DIN)
- new net: D448.2 (DOUT), D449.4 (DIN)
- new net: D447.2 (DOUT), D448.4 (DIN)
- new net: D1731.2 (DOUT), D1732.4 (DIN)
- new net: D1647.2 (DOUT), D1648.4 (DIN)
- new net: D446.2 (DOUT), D447.4 (DIN)
- new net: D2229.2 (DOUT), D2230.4 (DIN)
- new net: D2228.2 (DOUT), D2229.4 (DIN)
- new net: D438.2 (DOUT), D439.4 (DIN)
- new net: D1469.2 (DOUT), D1470.4 (DIN)
- new net: D698.2 (DOUT), D699.4 (DIN)
- new net: D1960.2 (DOUT), D1961.4 (DIN)
- new net: D185.2 (DOUT), D186.4 (DIN)
- new net: D184.2 (DOUT), D185.4 (DIN)
- new net: D1515.2 (DOUT), D1516.4 (DIN)
- new net: D1908.2 (DOUT), D1909.4 (DIN)
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
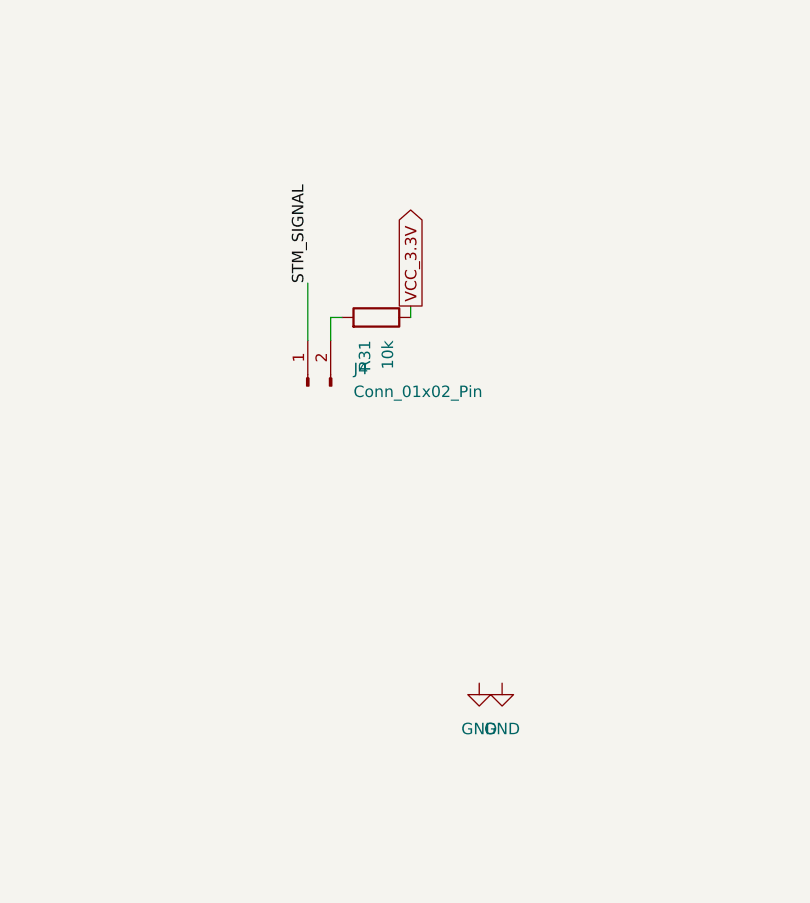
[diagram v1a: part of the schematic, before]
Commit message: .
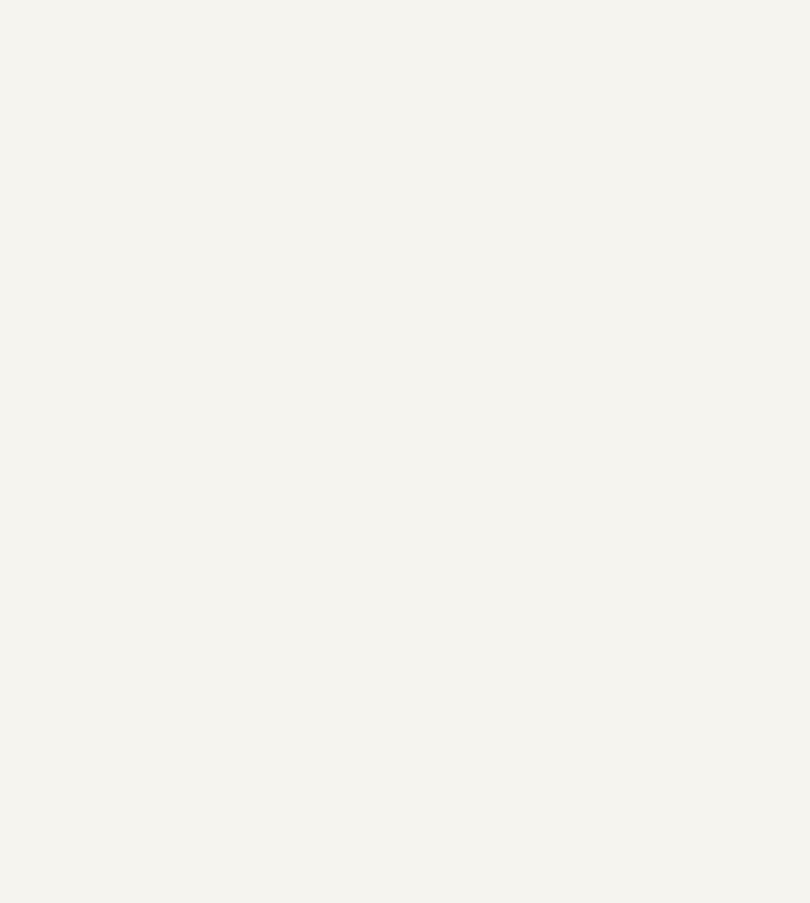
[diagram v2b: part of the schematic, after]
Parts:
- removed J4: Conn_01x02_Pin, Connector_JST:JST_EH_B2B-EH-A_1x02_P2.50mm_Vertical, symbol Connector:Conn_01x02_Pin
- removed R31: 10k, Resistor_SMD:R_0402_1005Metric, symbol Device:R
